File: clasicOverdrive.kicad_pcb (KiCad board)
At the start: 2 copper layers, 50 x 83 mm, 49 parts, among them CON1 SN49B12B, CON2 SN49B12B, J1 Jack-DC, Q1 2N2222, Q2 2N2222, U1 foot_switch, U2 LM4562

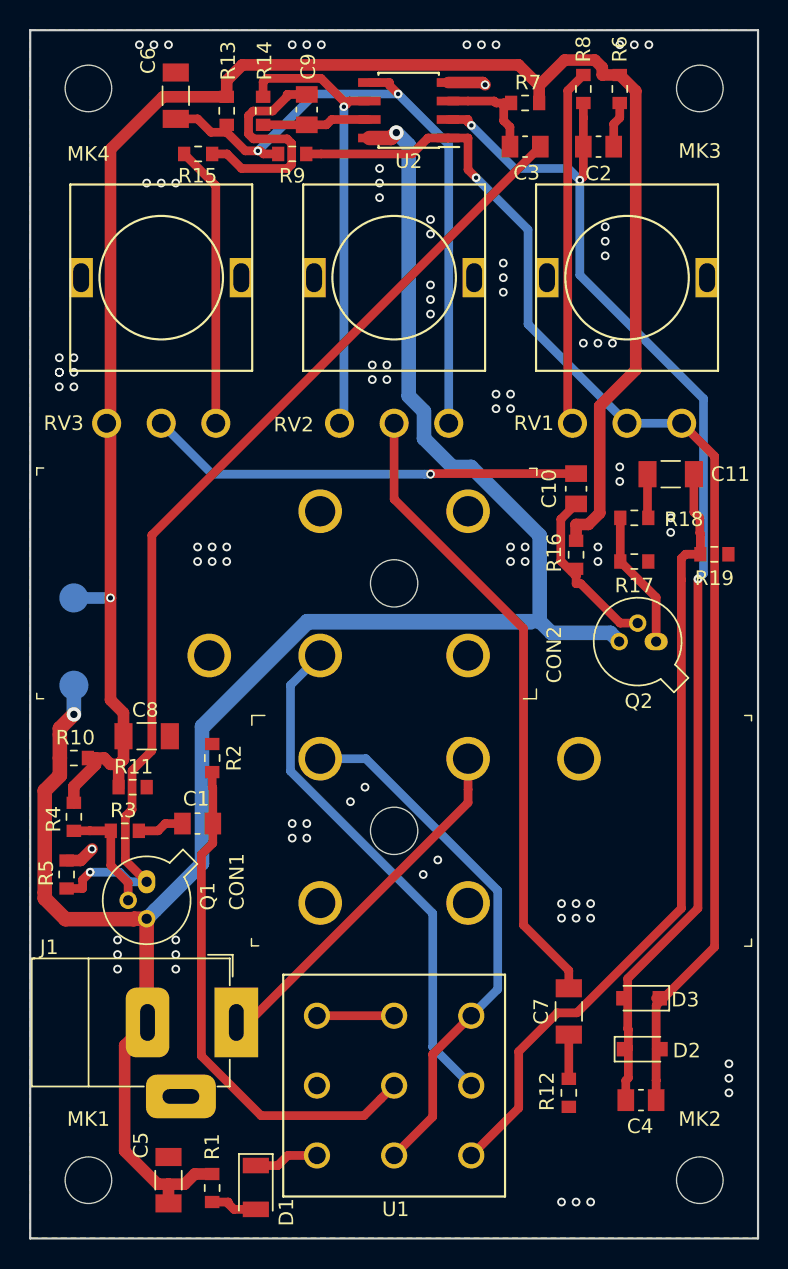
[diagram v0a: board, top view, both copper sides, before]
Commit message: Rev A
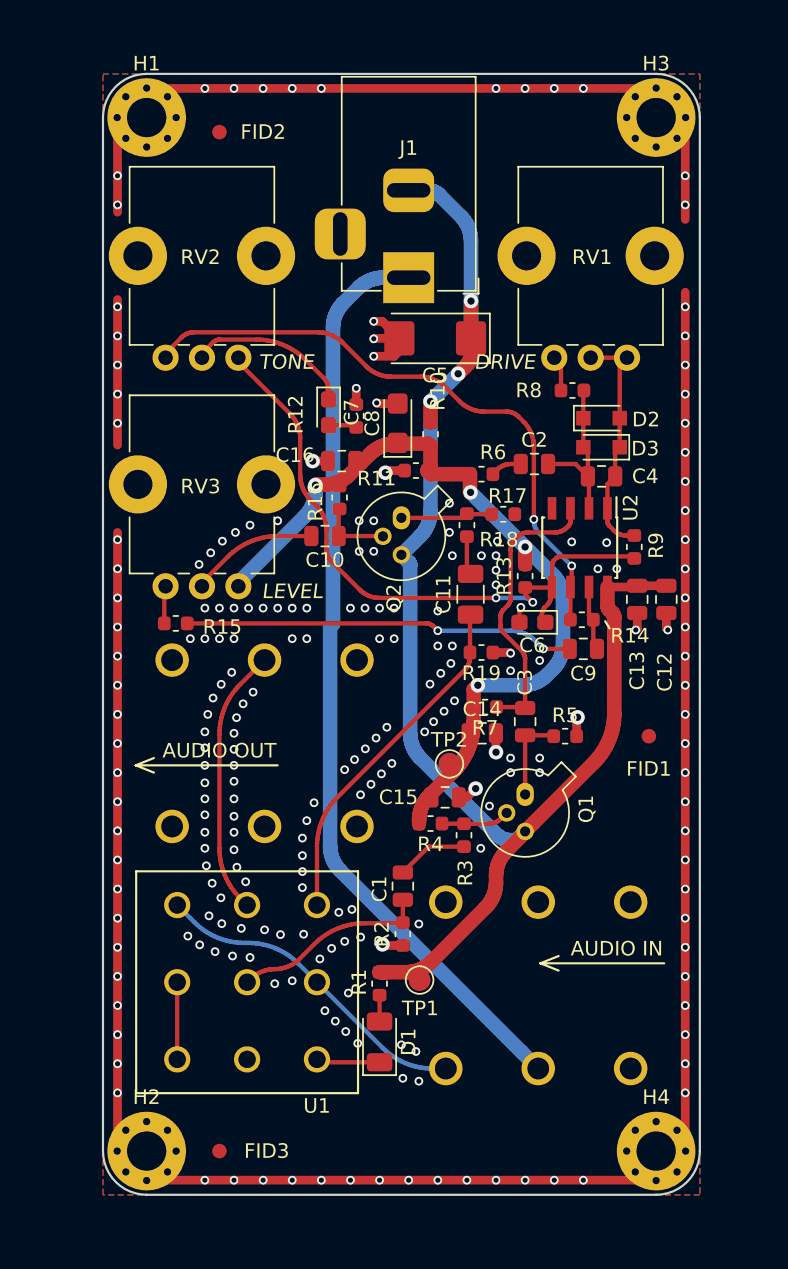
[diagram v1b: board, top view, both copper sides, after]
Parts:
- removed CON1, CON2: SN49B12B, digikey-footprints:Headphone_Jack_6.35mm_RA49B14B
- removed MK1, MK2, MK3, MK4: Mounting_Hole, MountingHole:MountingHole_3.2mm_M3
- added C12: 1u, Capacitor_SMD:C_0805_2012Metric, F.Cu at (143.7, 106.3)
- added C13: 0.1u, Capacitor_SMD:C_0805_2012Metric, F.Cu at (141.7, 106.3)
- added C14: 0.1u, Capacitor_SMD:C_0805_2012Metric, F.Cu at (131.1, 115.5)
- added C15: 0.1u, Capacitor_SMD:C_0805_2012Metric, F.Cu at (128.5, 119.9)
- added C16: 0.1u, Capacitor_SMD:C_0805_2012Metric, F.Cu at (121.4, 96.8)
- added FID1: Fiducial, Fiducial:Fiducial_1mm_Mask2mm, F.Cu at (142.5, 115.7)
- added FID2: Fiducial, Fiducial:Fiducial_1mm_Mask2mm, F.Cu at (113.0, 74.2)
- added FID3: Fiducial, Fiducial:Fiducial_1mm_Mask2mm, F.Cu at (113.0, 144.2)
- added H1: MountingHole_Pad, MountingHole:MountingHole_2.7mm_M2.5_Pad_Via, F.Cu at (108.0, 73.2)
- added H2: MountingHole_Pad, MountingHole:MountingHole_2.7mm_M2.5_Pad_Via, F.Cu at (108.0, 144.2)
- added H3: MountingHole_Pad, MountingHole:MountingHole_2.7mm_M2.5_Pad_Via, F.Cu at (143.0, 73.2)
- added H4: MountingHole_Pad, MountingHole:MountingHole_2.7mm_M2.5_Pad_Via, F.Cu at (143.0, 144.2)
- added J2: AudioJack3_Switch, clasicOverdrive:Jack_6.35mm_Amphenol_ACJS-MHOM, B.Cu at (146.0, 131.3)
- added J3: AudioJack3_Switch, clasicOverdrive:Jack_6.35mm_Amphenol_ACJS-MHOM, B.Cu at (105.0, 117.7)
- added T1: LA_LOGO, clasicOverdrive:LA_LOGO_MASK, F.Cu at (123.5, 145.2)
- C1, C10, C2, C3, C4, C9: footprint Capacitor_SMD:C_0805_2012Metric_Pad1.15x1.50mm_HandSolder -> Capacitor_SMD:C_0805_2012Metric
- C11: footprint Capacitor_SMD:C_1206_3216Metric_Pad1.24x1.80mm_HandSolder -> Capacitor_SMD:C_1206_3216Metric
- C5: footprint Capacitor_SMD:C_1206_3216Metric_Pad1.24x1.80mm_HandSolder -> Capacitor_Tantalum_SMD:CP_EIA-6032-28_Kemet-C
- C6, C7: footprint Capacitor_SMD:C_1206_3216Metric_Pad1.24x1.80mm_HandSolder -> Capacitor_Tantalum_SMD:CP_EIA-2012-12_Kemet-R
- C8: footprint Capacitor_SMD:C_1206_3216Metric_Pad1.24x1.80mm_HandSolder -> Capacitor_Tantalum_SMD:CP_EIA-3216-18_Kemet-A
- D1: footprint LED_SMD:LED_1206_3216Metric_Pad1.07x1.80mm_HandSolder -> LED_SMD:LED_1206_3216Metric
- J1: footprint Connector_Audio:Jack_Horizontal -> Connector_BarrelJack:BarrelJack_Horizontal
- R1, R10, R11, R12, R13, R14, R15, R16, R17, R18, R19, R2, R3, R4, R5, R6, R7, R8, R9: footprint Resistor_SMD:R_0603_1608Metric_Pad0.84x1.00mm_HandSolder -> Resistor_SMD:R_0603_1608Metric
- RV1, RV2, RV3: footprint clasicOverdrive:Pot_series_296 -> Potentiometer_THT:Potentiometer_Bourns_PTV09A-1_Single_Vertical
- TP1, TP2: footprint TestPoint:TestPoint_Pad_D2.0mm -> TestPoint:TestPoint_Pad_D1.5mm; moved to F.Cu
- U1: footprint clasicOverdrive:FS57003PLT2B2M2QE -> clasicOverdrive:Foot_Switch_E-Switch_FS57003PLT2B2M2QE
- moved C5 60.7 mm to (127.9, 88.4), turned to 180 degrees
- moved J1 52.5 mm to (126.0, 84.2), turned to 270 degrees
- moved R12 48.7 mm to (122.4, 93.7), turned to 90 degrees
- moved C7 44.3 mm to (120.5, 93.5)
- moved C6 43.7 mm to (134.5, 107.9), turned to 180 degrees
- moved D2 43.4 mm to (139.3, 93.9)
- moved C4 42.9 mm to (139.3, 97.9)
- moved C9 41.6 mm to (138.0, 109.7), turned to 0 degrees
- moved R7 41.6 mm to (131.3, 113.7), turned to 180 degrees
- moved R14 41.3 mm to (137.9, 107.7), turned to 180 degrees
- moved C3 39.5 mm to (134.0, 114.7), turned to 270 degrees
- moved R13 38.0 mm to (134.0, 104.7)
- moved D3 37.9 mm to (139.3, 95.9)
- moved R9 35.8 mm to (141.5, 102.7), turned to 90 degrees
- moved R5 35.5 mm to (136.8, 115.7), turned to 0 degrees
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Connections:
- J1 pad 1: Net-(CON1-PadR) -> GNDPWR
- RV1 pad 1: Net-(R8-Pad1) -> Net-(C4-Pad2)
- RV1 pad 3: Net-(C4-Pad2) -> Net-(R8-Pad1)
- RV2 pad 1: Net-(R14-Pad2) -> Net-(C6-Pad1)
- RV2 pad 3: Net-(C6-Pad1) -> Net-(R14-Pad2)
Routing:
- net GND: track 4.69 -> 230.6 mm, vias 92 -> 227
- net Net-(C2-Pad2): track 85.3 -> 11.4 mm, vias 3 -> 0
- net +9V: track 173.0 -> 99.4 mm, vias 2 -> 3
- net Net-(C4-Pad2): track 89.1 -> 16.6 mm, vias 1 -> 0
- net +4V5: track 129.0 -> 56.7 mm, vias 1 -> 4
- net GNDPWR: track 0.00 -> 64.4 mm
- net Net-(C3-Pad2): track 69.5 -> 6.05 mm, vias 1 -> 0
- net Net-(C7-Pad1): track 43.8 -> 11.1 mm
- net Net-(C11-Pad2): track 54.9 -> 24.1 mm
- net Net-(CON1-PadR): track 25.2 -> 0.00 mm
- net Net-(R8-Pad1): track 24.5 -> 2.44 mm
- net Net-(C1-Pad2): track 35.6 -> 13.6 mm
- net Net-(C10-Pad2): track 30.0 -> 9.05 mm, vias 1 -> 0
- net Net-(J3-PadR): track 35.5 -> 18.5 mm
- net Net-(R15-Pad1): track 19.4 -> 2.59 mm
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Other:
- board size 50 x 83 mm -> 41 x 77 mm
- net class Default: trace_width 0.6 -> 0.3
- net class PWR: trace_width 0.8 -> 0.6; via_dia 0.6 -> 1; via_drill 0.35 -> 0.5
- rule pad_to_mask_clearance: 0.2 -> 0
- rule solder_mask_min_width: 0.25 -> 0.1
- board text added: "AUDIO IN"
- board text added: "AUDIO OUT"
- board text added: "Rev: A 2019/11/30 clasicOverdrive"
